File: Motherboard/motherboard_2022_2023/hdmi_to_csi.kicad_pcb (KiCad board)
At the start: 2 copper layers, 17.1 x 29.2 mm, 4 parts, among them J15 Conn_01x22_Shielded, J16 HDMI_C_1.4

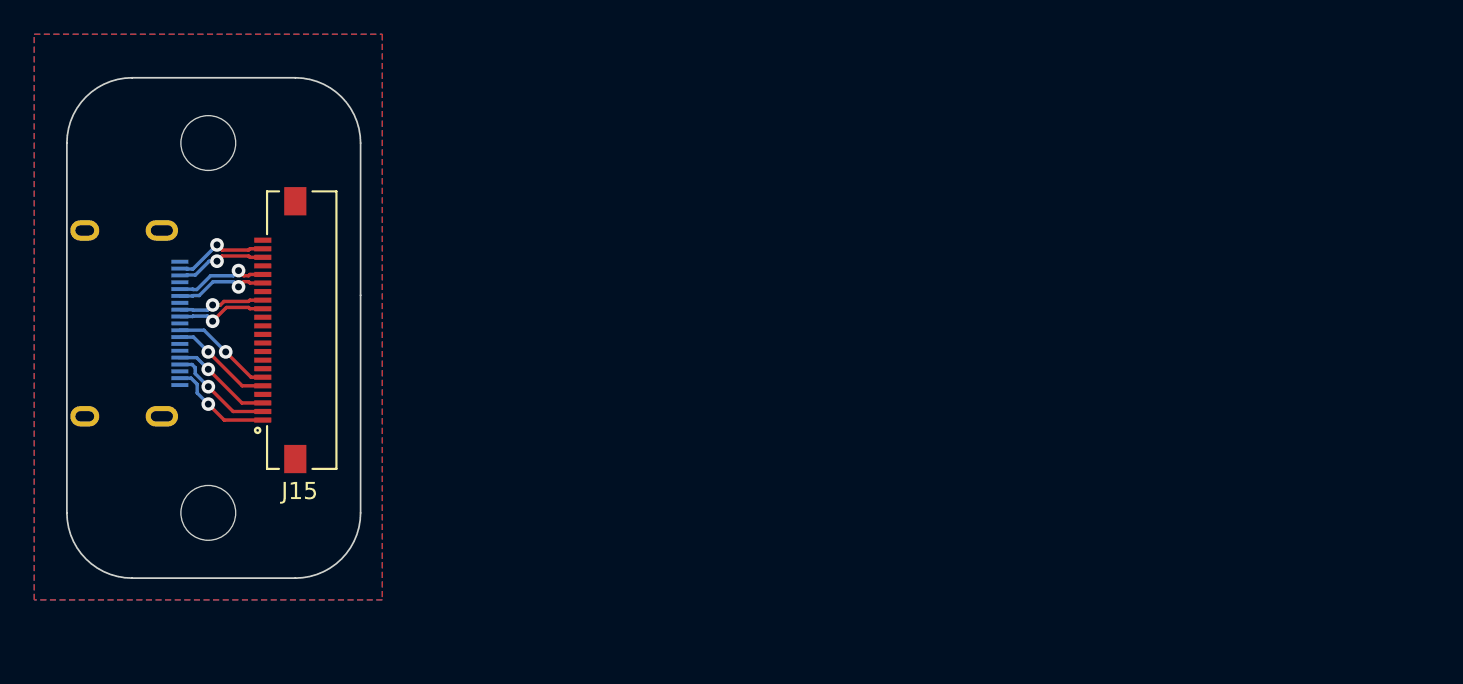
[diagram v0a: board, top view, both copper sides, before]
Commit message: Updated Both PCBs
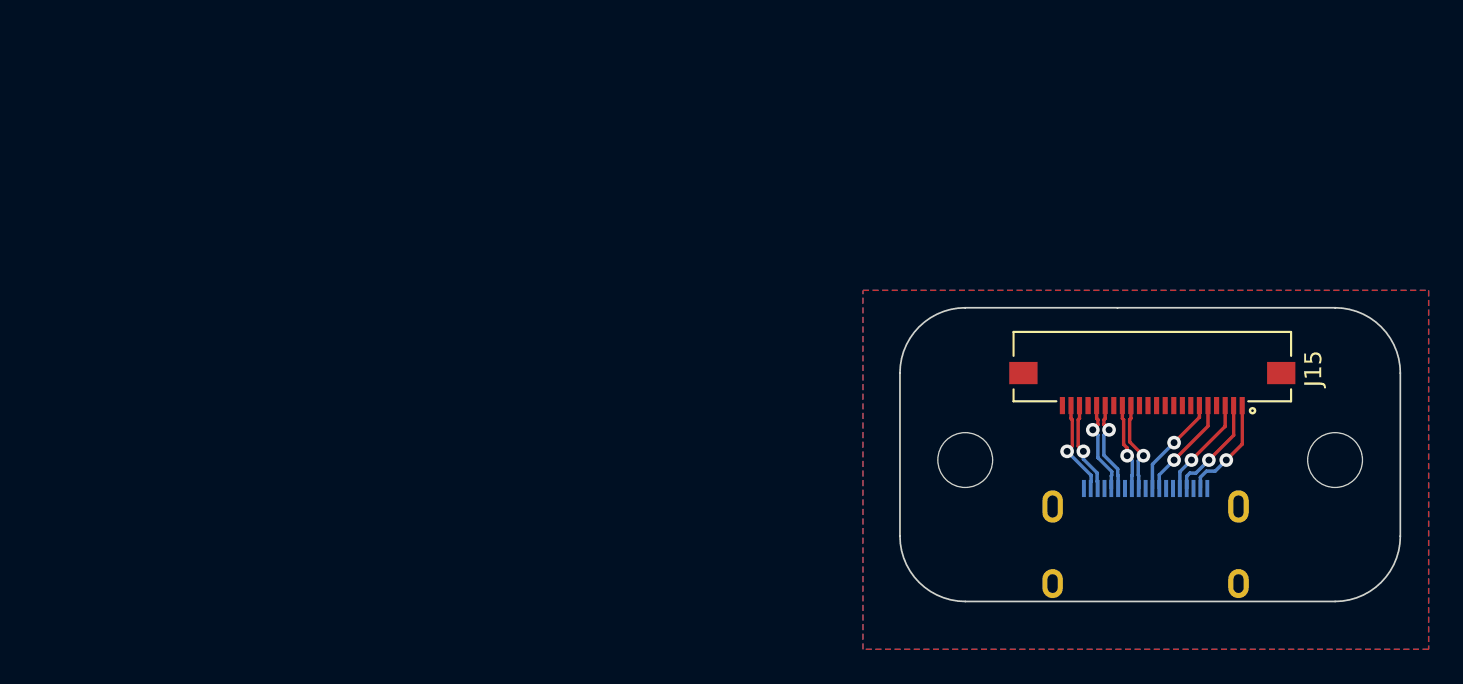
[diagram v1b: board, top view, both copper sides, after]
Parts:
- moved H5 65.8 mm to (155.7, 105.6), turned to 0 degrees
- moved J16 57.2 mm to (144.6, 107.3), turned to 180 degrees
- moved J15 52.1 mm to (145.0, 102.4), turned to 180 degrees
- moved H6 47.9 mm to (134.1, 105.6), turned to 0 degrees
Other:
- board size 17.1 x 29.2 mm -> 29.2 x 17.1 mm
